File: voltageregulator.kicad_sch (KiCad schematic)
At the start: 36 parts, among them Q1 Si2319CDS, U1 LM317_SOT-223, U2 LM337_SOT223, U3 TPS65131RGE

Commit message: Added new branch. New branch for different +-9V power supply.
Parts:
- D1, D2: footprint Diode_SMD:D_Powermite_AK -> Diode_SMD:D_Powermite_LargeCathode
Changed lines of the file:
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@@
 	)
 	(junction
+		(at 157.48 71.12)
+		(diameter 0)
+		(color 0 0 0 0)
+	)
+	(junction
 		(at 88.9 114.3)
 		(diameter 0)
@@
 	)
 	(junction
-		(at 124.46 38.1)
+		(at 99.06 38.1)
 		(diameter 0)
 		(color 0 0 0 0)
@@
 	)
 	(junction
-		(at 99.06 38.1)
+		(at 203.2 66.04)
 		(diameter 0)
 		(color 0 0 0 0)
 	)
 	(junction
-		(at 203.2 66.04)
+		(at 124.46 38.1)
 		(diameter 0)
 		(color 0 0 0 0)
@@
 	)
 	(junction
-		(at 157.48 71.12)
-		(diameter 0)
-		(color 0 0 0 0)
-	)
-	(junction
 		(at 88.9 165.1)
 		(diameter 0)
@@
 	(wire
 		(pts
-			(xy 99.06 38.1) (xy 106.68 38.1)
-		)
-		(stroke
-			(width 0)
-			(type default)
-		)
-	)
-	(wire
-		(pts
 			(xy 71.12 152.4) (xy 88.9 152.4)
 		)
@@
 	(wire
 		(pts
-			(xy 124.46 50.8) (xy 124.46 38.1)
+			(xy 124.46 19.05) (xy 124.46 38.1)
 		)
 		(stroke
@@
 	(wire
 		(pts
-			(xy 177.8 71.12) (xy 172.72 71.12)
+			(xy 167.64 20.32) (xy 167.64 19.05)
 		)
 		(stroke
@@
 	(wire
 		(pts
-			(xy 167.64 20.32) (xy 167.64 19.05)
+			(xy 71.12 157.48) (xy 71.12 152.4)
 		)
 		(stroke
@@
 	(wire
 		(pts
-			(xy 71.12 157.48) (xy 71.12 152.4)
+			(xy 133.35 55.88) (xy 137.16 55.88)
 		)
 		(stroke
@@
 	(wire
 		(pts
-			(xy 133.35 55.88) (xy 137.16 55.88)
+			(xy 88.9 63.5) (xy 100.33 63.5)
 		)
 		(stroke
@@
 	(wire
 		(pts
-			(xy 88.9 63.5) (xy 100.33 63.5)
+			(xy 172.72 71.12) (xy 177.8 71.12)
 		)
 		(stroke
@@
 	(wire
 		(pts
-			(xy 157.48 71.12) (xy 165.1 71.12)
-		)
-		(stroke
-			(width 0)
-			(type default)
-		)
-	)
-	(wire
-		(pts
 			(xy 156.21 48.26) (xy 152.4 48.26)
 		)
@@
 	(wire
 		(pts
+			(xy 157.48 71.12) (xy 165.1 71.12)
+		)
+		(stroke
+			(width 0)
+			(type default)
+		)
+	)
+	(wire
+		(pts
 			(xy 133.35 48.26) (xy 133.35 55.88)
 		)
@@
 	(wire
 		(pts
-			(xy 124.46 19.05) (xy 124.46 38.1)
+			(xy 114.3 38.1) (xy 124.46 38.1)
 		)
 		(stroke
@@
 	(wire
 		(pts
+			(xy 106.68 38.1) (xy 99.06 38.1)
+		)
+		(stroke
+			(width 0)
+			(type default)
+		)
+	)
+	(wire
+		(pts
 			(xy 50.8 114.3) (xy 50.8 123.19)
 		)
@@
 	(wire
 		(pts
-			(xy 63.5 63.5) (xy 74.93 63.5)
+			(xy 124.46 38.1) (xy 124.46 50.8)
 		)
 		(stroke
@@
 	(wire
 		(pts
-			(xy 63.5 68.58) (xy 63.5 63.5)
+			(xy 63.5 63.5) (xy 74.93 63.5)
 		)
 		(stroke
@@
 	(wire
 		(pts
-			(xy 114.3 38.1) (xy 124.46 38.1)
+			(xy 63.5 68.58) (xy 63.5 63.5)
 		)
 		(stroke
@@
 			)
 		)
-		(property "Footprint" "Diode_SMD:D_Powermite_AK"
+		(property "Footprint" "Diode_SMD:D_Powermite_LargeCathode"
 			(at 168.91 75.565 0)
 			(hide yes)
@@
 			)
 		)
-		(property "Footprint" "Diode_SMD:D_Powermite_AK"
+		(property "Footprint" "Diode_SMD:D_Powermite_LargeCathode"
 			(at 110.49 33.655 0)
 			(hide yes)

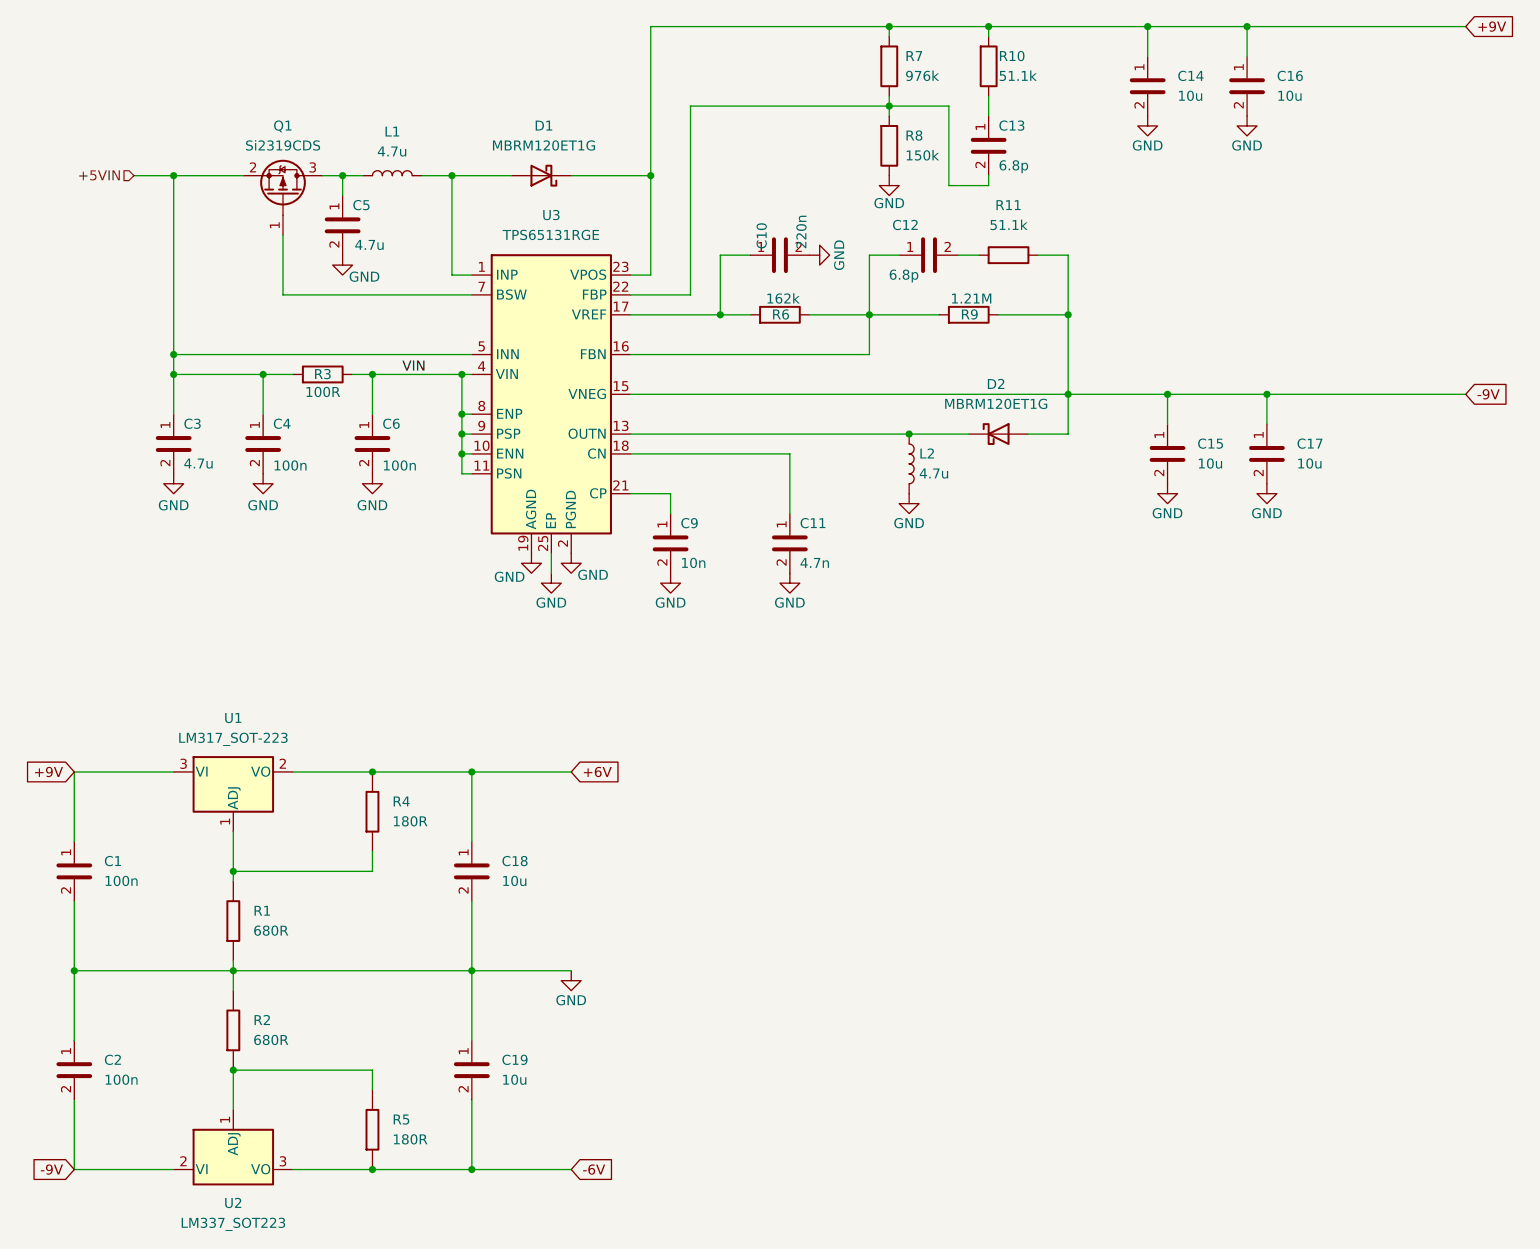
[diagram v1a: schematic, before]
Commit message: Save progress.
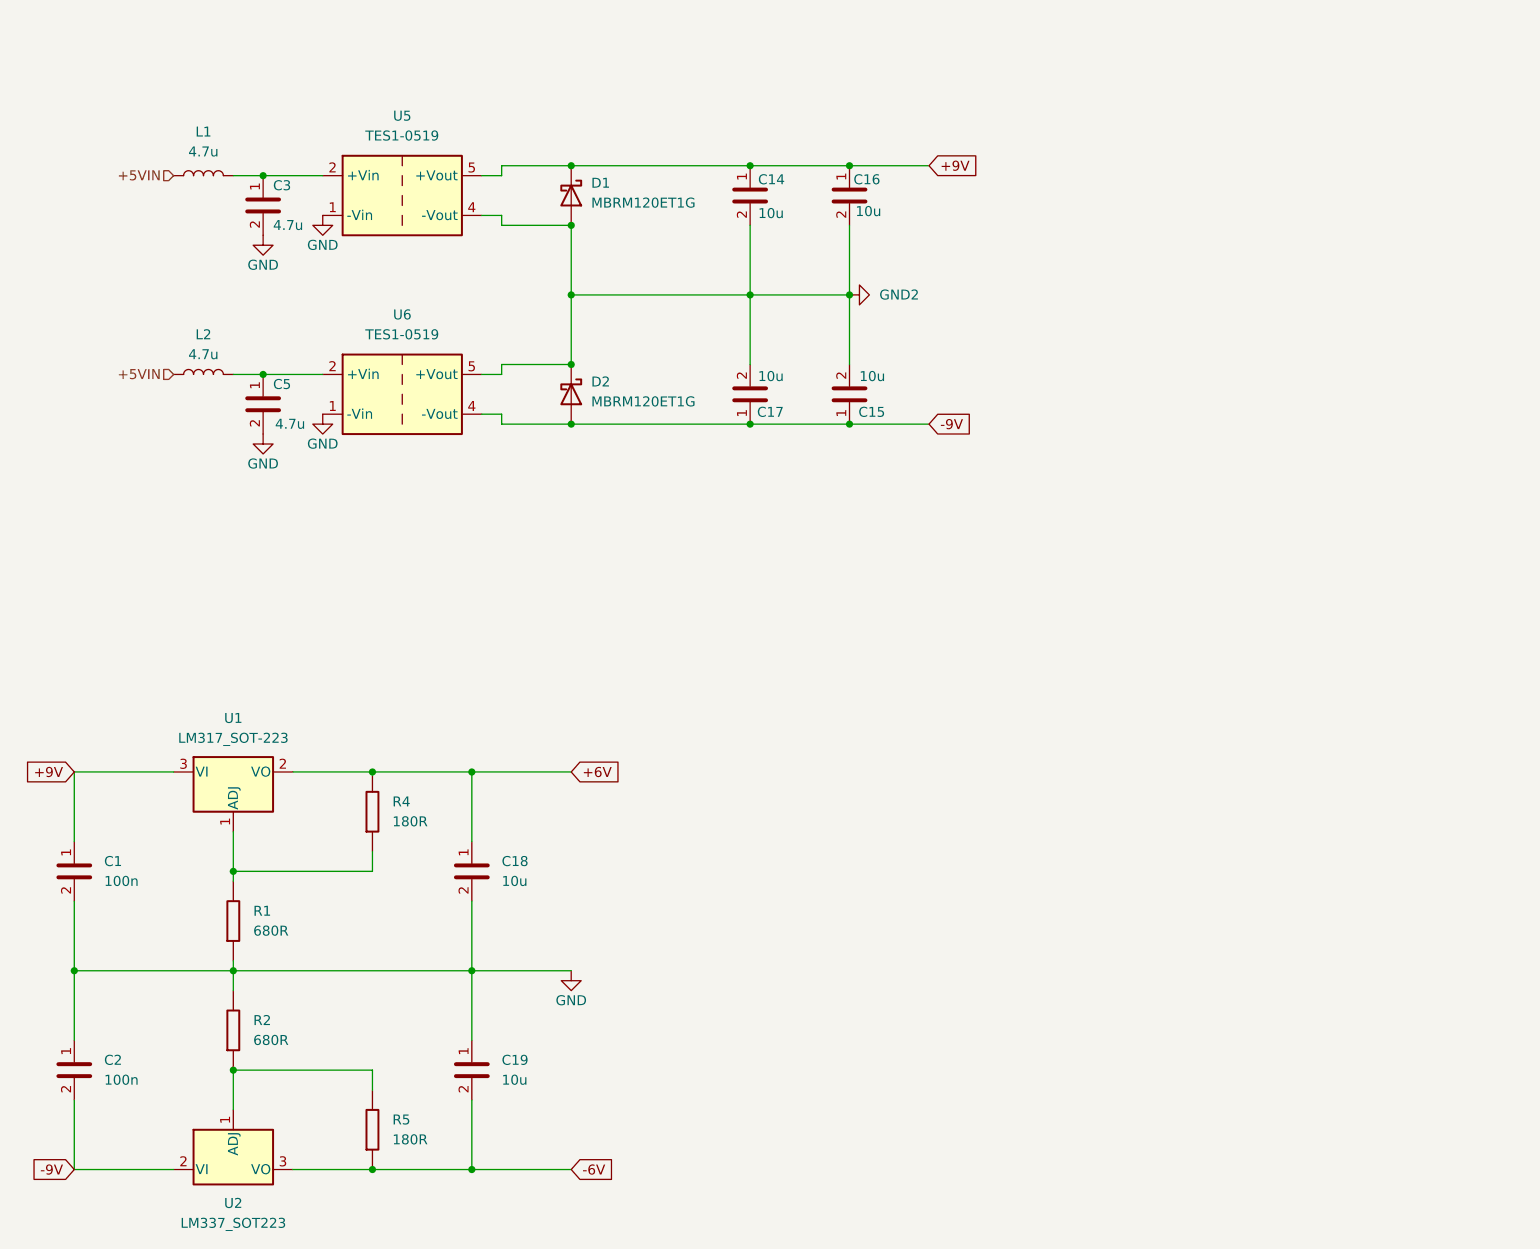
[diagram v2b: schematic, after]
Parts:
- removed C10: 220n, Capacitor_SMD:C_0402_1005Metric_Pad0.74x0.62mm_HandSolder, symbol 1_C_SMD:C_0402_220n_25V
- removed C11: 4.7n, Capacitor_SMD:C_0402_1005Metric_Pad0.74x0.62mm_HandSolder, symbol 1_C_SMD:C_0402_4.7n_25V
- removed C12, C13: 6.8p, Capacitor_SMD:C_0402_1005Metric_Pad0.74x0.62mm_HandSolder, symbol 1_C_SMD:C_0402_6.8p_25V
- removed C4, C6: 100n, Capacitor_SMD:C_0402_1005Metric_Pad0.74x0.62mm_HandSolder, symbol 1_C_SMD:C_0402_100n_25V
- removed C9: 10n, Capacitor_SMD:C_0402_1005Metric_Pad0.74x0.62mm_HandSolder, symbol 1_C_SMD:C_0402_10n_25V
- removed Q1: Si2319CDS, Package_TO_SOT_SMD:SOT-23, symbol Transistor_FET:Si2319CDS
- removed R10, R11: 51.1k, Resistor_SMD:R_0402_1005Metric_Pad0.72x0.64mm_HandSolder, symbol 1_R_SMD:R_0402_51.1k
- removed R3: 100R, Resistor_SMD:R_0402_1005Metric_Pad0.72x0.64mm_HandSolder, symbol 1_R_SMD:R_0402_100R
- removed R6: 162k, Resistor_SMD:R_0402_1005Metric_Pad0.72x0.64mm_HandSolder, symbol 1_R_SMD:R_0402_162k
- removed R7: 976k, Resistor_SMD:R_0402_1005Metric_Pad0.72x0.64mm_HandSolder, symbol 1_R_SMD:R_0402_976k
- removed R8: 150k, Resistor_SMD:R_0402_1005Metric_Pad0.72x0.64mm_HandSolder, symbol 1_R_SMD:R_0402_150k
- removed R9: 1.21M, Resistor_SMD:R_0402_1005Metric_Pad0.72x0.64mm_HandSolder, symbol 1_R_SMD:R_0402_1.21M
- removed U3: TPS65131RGE, Package_DFN_QFN:VQFN-24-1EP_4x4mm_P0.5mm_EP2.45x2.45mm_ThermalVias, symbol Regulator_Switching:TPS65131RGE
- added U5, U6: TES1-0519, Converter_DCDC:Converter_DCDC_TRACO_TES1-051x_121x_241x_Single_SMD, symbol Converter_DCDC:TES1-0519
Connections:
- net +5VIN: now also L1.1, L2.1; no longer C3.1
- net +9V: now also U5.5 (+Vout)
- net -9V: now also U6.4 (-Vout)
- net GND: now also U5.1 (-Vin), U6.1 (-Vin); no longer C14.2, C15.2, C16.2, C17.2, L2.2
- net GND2: now reaches D2.1 (K)
- net GND2: now also C14.2, C15.2, C16.2, C17.2, D1.2 (A), U5.4 (-Vout), U6.5 (+Vout); no longer L2.1
- net at C5.1: now also L2.2, U6.2 (+Vin); no longer L1.1
- net at L1.2: now also C3.1, U5.2 (+Vin); no longer D1.2 (A)
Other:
- moved on the sheet: C14, C15, C16, C17, C3, C5, D1, D2, L1, L2

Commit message: Save progress.
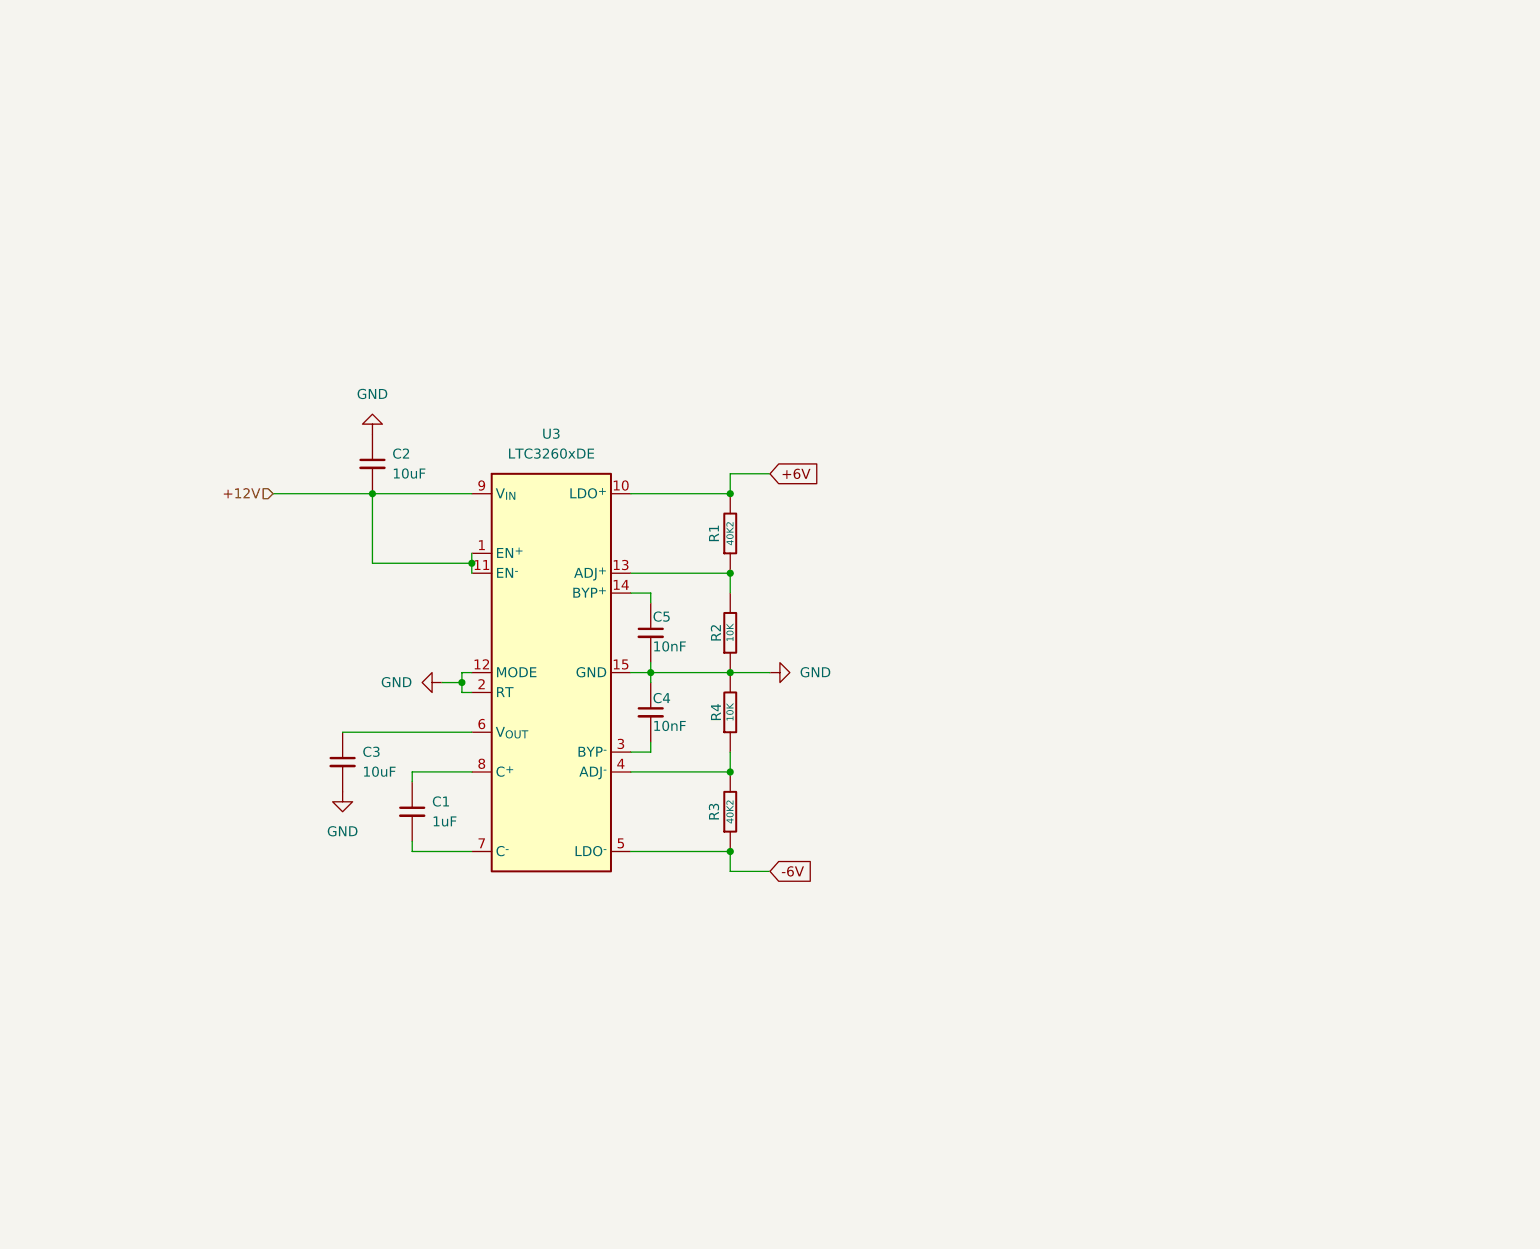
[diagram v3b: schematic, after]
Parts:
- removed C1, C2: 100n, Capacitor_SMD:C_0402_1005Metric_Pad0.74x0.62mm_HandSolder, symbol 1_C_SMD:C_0402_100n_25V
- removed C14, C15, C16, C17, C18, C19: 10u, Capacitor_SMD:C_0603_1608Metric_Pad1.08x0.95mm_HandSolder, symbol 1_C_SMD:C_0603_10u
- removed C3, C5: 4.7u, Capacitor_SMD:C_0402_1005Metric_Pad0.74x0.62mm_HandSolder, symbol 1_C_SMD:C_0402_4.7u_10V
- removed D1, D2: MBRM120ET1G, Diode_SMD:D_Powermite_LargeCathode, symbol 1_Diode_SMD:MBRM120ET1G
- removed L1, L2: 4.7u, 1_L_SMD:L_Bourns_SRP4021HMT, symbol Device:L
- removed R1, R2: 680R, Resistor_SMD:R_0603_1608Metric_Pad0.98x0.95mm_HandSolder, symbol DK_Yageo_0603_Resistors_E96_1%_100mW_ThinFilm:R_680R
- removed R4, R5: 180R, Resistor_SMD:R_0603_1608Metric_Pad0.98x0.95mm_HandSolder, symbol DK_Yageo_0603_Resistors_E96_1%_100mW_ThinFilm:R_240R
- removed U1: LM317_SOT-223, Package_TO_SOT_SMD:SOT-223-3_TabPin2, symbol Regulator_Linear:LM317_SOT-223
- removed U2: LM337_SOT223, Package_TO_SOT_SMD:SOT-223-3_TabPin2, symbol Regulator_Linear:LM337_SOT223
- removed U5, U6: TES1-0519, Converter_DCDC:Converter_DCDC_TRACO_TES1-051x_121x_241x_Single_SMD, symbol Converter_DCDC:TES1-0519
- added C1: 1uF, Capacitor_SMD:C_0402_1005Metric_Pad0.74x0.62mm_HandSolder, symbol DK_Murata_GRM_0402_Capacitors:C_1uF_2
- added C2, C3: 10uF, Capacitor_SMD:C_0603_1608Metric_Pad1.08x0.95mm_HandSolder, symbol DK_Murata_GRM_0603_Capacitors:C_10uF_16
- added C4, C5: 10nF, Capacitor_SMD:C_0402_1005Metric_Pad0.74x0.62mm_HandSolder, symbol DK_Murata_GRM_0402_Capacitors:C_10nF_2
- added R1, R3: 40K2, Resistor_SMD:R_0402_1005Metric_Pad0.72x0.64mm_HandSolder, symbol DK_Yageo_RC_0402_Resistors:R_40K2
- added R2, R4: 10K, Resistor_SMD:R_0402_1005Metric_Pad0.72x0.64mm_HandSolder, symbol DK_Yageo_0402_Resistors_1%_63mW_ThinFilm:R_10K
- added U3: LTC3260xDE, Package_DFN_QFN:DFN-14-1EP_3x4mm_P0.5mm_EP1.7x3.3mm, symbol Regulator_SwitchedCapacitor:LTC3260xDE
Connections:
- net +6V: now also R1.2, U3.10 (LDO^{+})
- net -6V: now also R3.1, U3.5 (LDO^{-})
- net GND: now also C2.1, C3.2, C4.1, C5.2, R2.1, R4.2, U3.12 (MODE), U3.15 (GND), U3.2 (RT)
- new net: R1.1, R2.2, U3.13 (ADJ^{+})
- new net: R3.2, R4.1, U3.4 (ADJ^{-})
- new net: C3.1, U3.6 (V_{OUT})
- new net: C1.1, U3.8 (C^{+})
- new net: C1.2, U3.7 (C^{-})
- new net: C5.1, U3.14 (BYP^{+})
- new net: C4.2, U3.3 (BYP^{-})
- new net +12V: C2.2, U3.1 (EN^{+}), U3.11 (EN^{-}), U3.9 (V_{IN})

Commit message: Added fabrication files. Board finalized.
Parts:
- U3: DigiKey Part Number (none) -> LTC3260EDE#TRPBFTR-ND; Manufacturer (none) -> Analog Devices Inc.; Manufacturer Part Number (none) -> LTC3260EDE#TRPBF; Package/Footprint (none) -> DFN-14; Type (none) -> SMD
